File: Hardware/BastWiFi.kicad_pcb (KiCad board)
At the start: 2 copper layers, 60 x 22.9 mm, 37 parts, among them J1 Conn_Battery, J3 Conn_Left, J4 Conn_Right, P1 USB_C_Plug_USB2.0, Q1 DMG3415U-7, SW1 GPIO0, SW2 RESET, U1 MCP73831-3-OT, U2 AP2112K-3.3, U3 ESP32-S2-WROVER

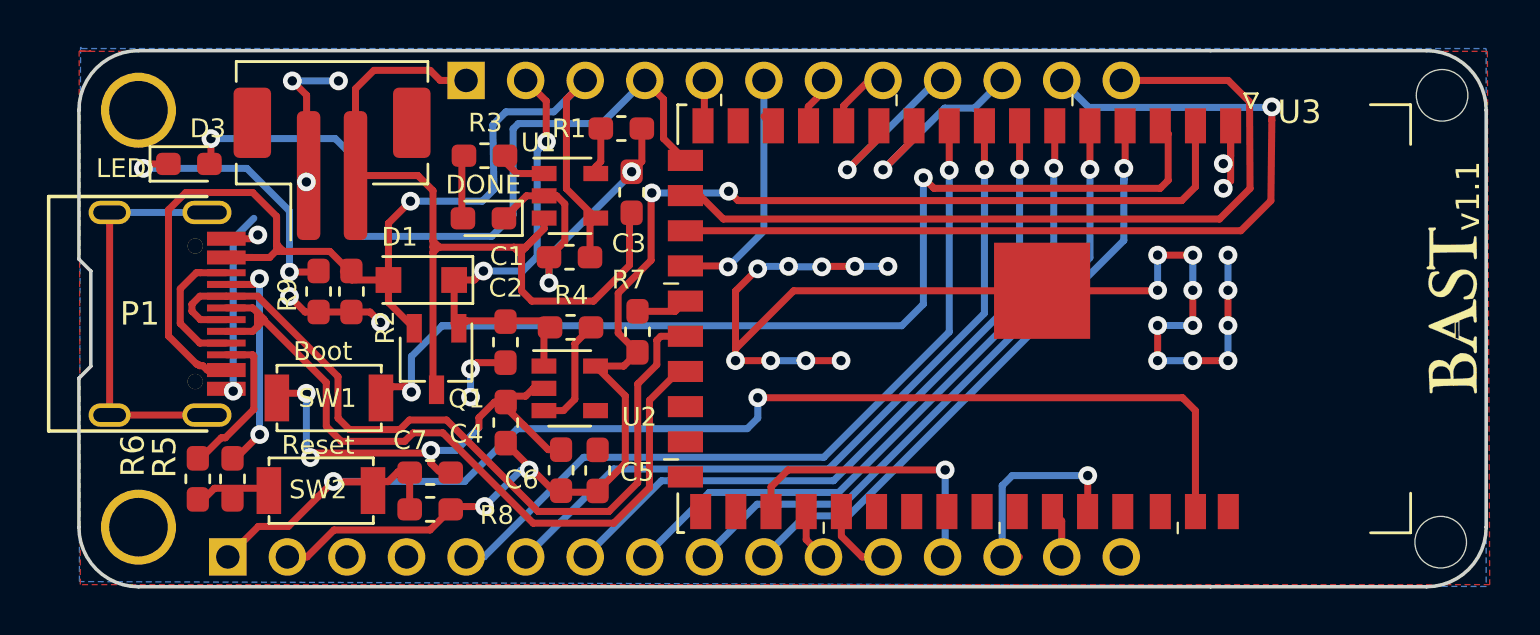
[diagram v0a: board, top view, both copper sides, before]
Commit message: change pads
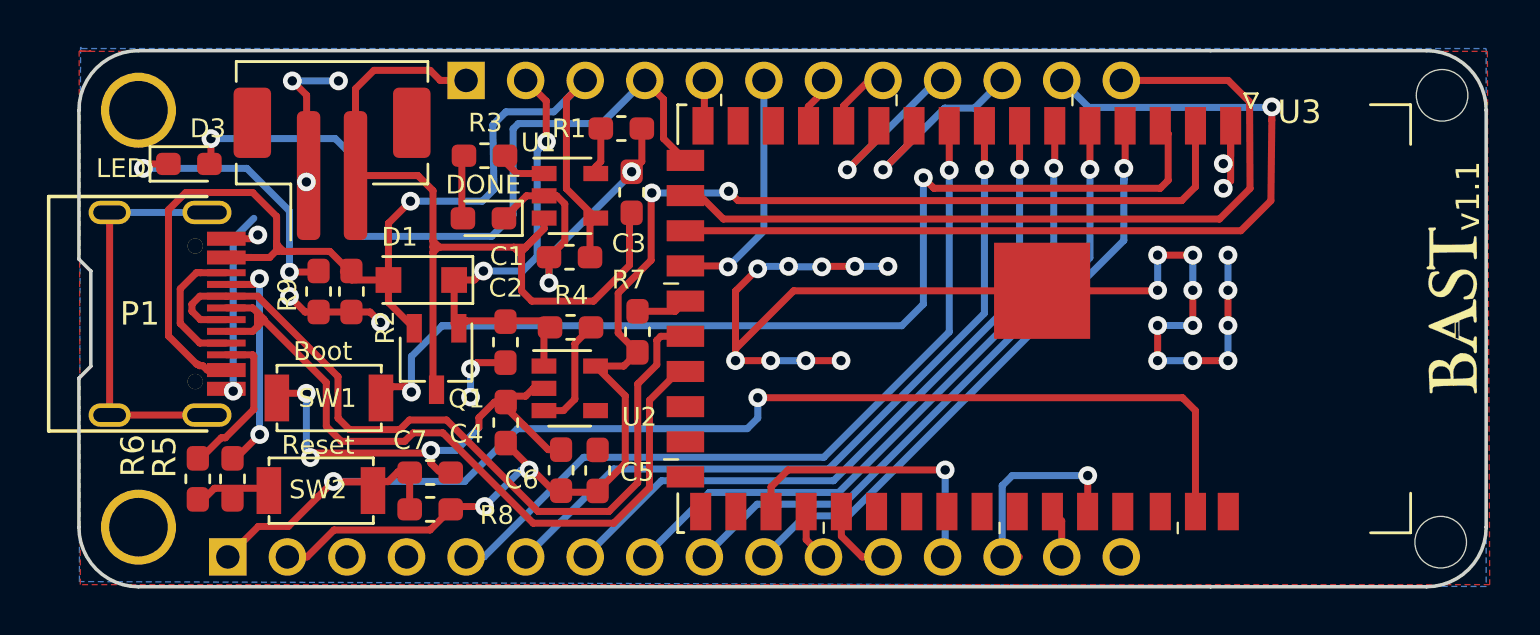
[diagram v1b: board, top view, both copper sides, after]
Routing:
- net Net-(U3-Pad14): track 0.57 -> 0.00 mm
